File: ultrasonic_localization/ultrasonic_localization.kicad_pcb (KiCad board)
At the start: 2 copper layers, 69.6 x 80.4 mm, 212 parts, among them J101 USB_OTG_fix, J102 Conn_02x03_Odd_Even, J401 Screw_Terminal_1x02_Bat, Q101 BUK9Y29-40E, Q301 BC847, Q501 BC847, Q601 BC847, Q701 BC847, SW101 SW_Push, SW102 SW_DPDT, SW103 SW_DPDT, U101 ATMEGA32U4RC-AU, U102 MD0105, U103 4047, U201 nRF24L01+, U202 ANT016008LCS2442MA2, U301 LM324, U302 TCT40-16R/T, U401 AP3012, U402 AP3012, U403 TPS6223x, U404 LP5907SNX-3.3/NOPB, U405 BQ2423, U501 LM324, U502 TCT40-16R/T, U601 LM324, U602 TCT40-16R/T, U701 LM324, U702 TCT40-16R/T, U801 IMU, U802 Level_Shifter_4Channel, Y101 Crystal_GND24, Y201 16MHz

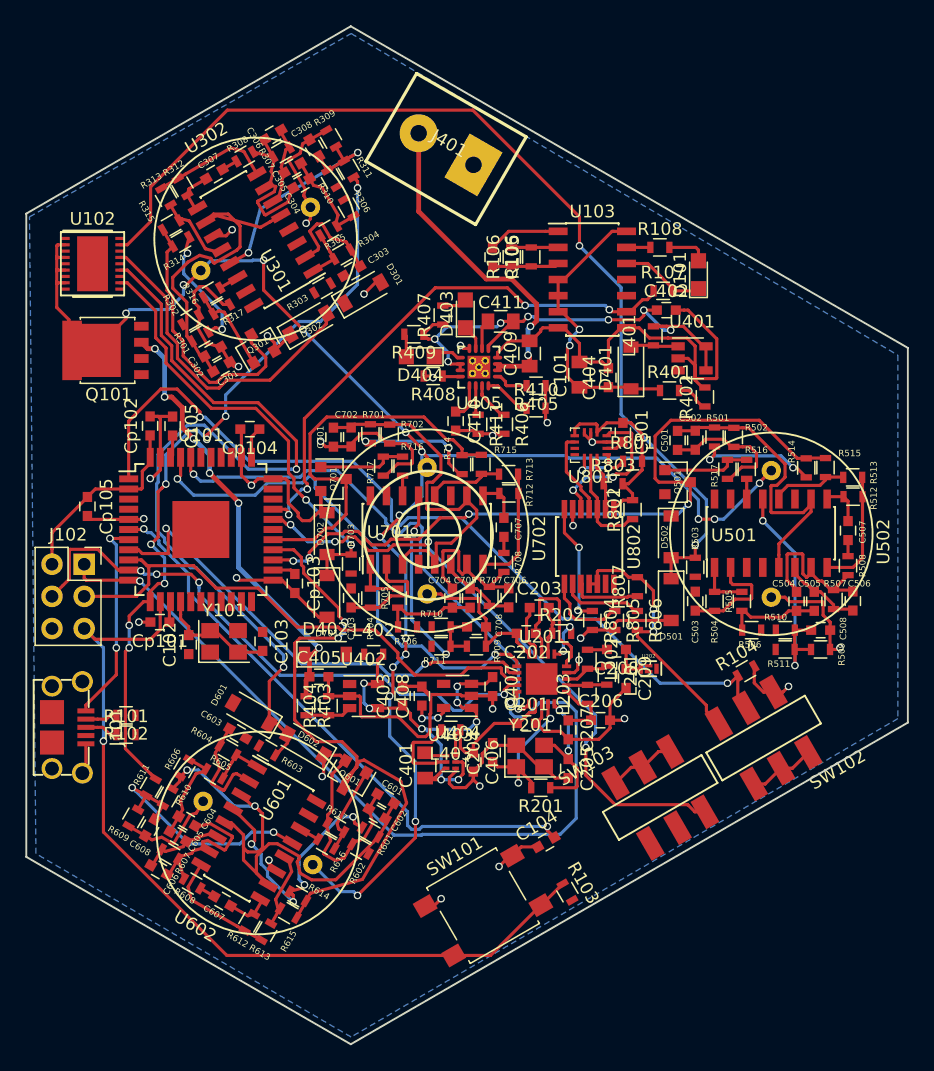
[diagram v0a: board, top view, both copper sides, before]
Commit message: Finished routing
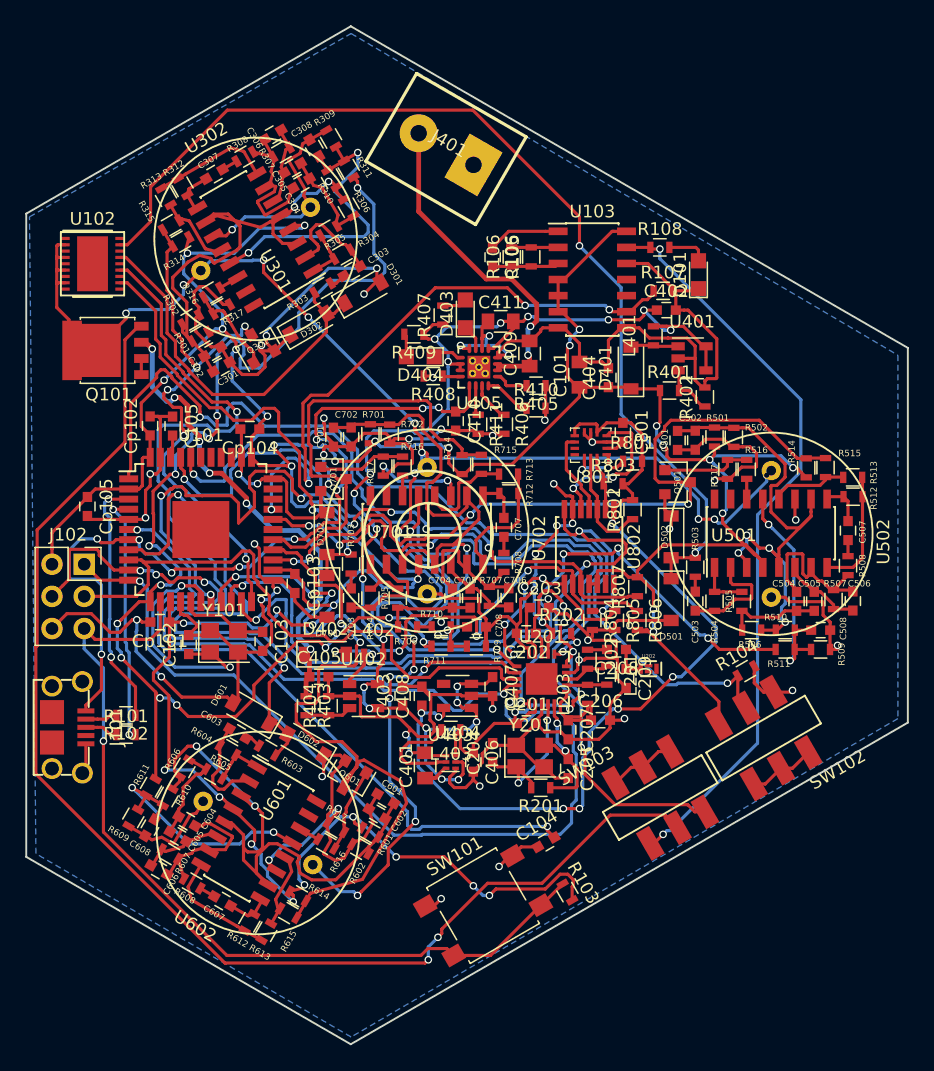
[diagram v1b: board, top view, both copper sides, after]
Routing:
- net +5V: track 117.0 -> 297.4 mm, vias 14 -> 34
- net GND: track 295.5 -> 438.4 mm, vias 28 -> 52
- net Net-(Q101-Pad4): track 0.00 -> 101.9 mm, vias 0 -> 2
- net /THRESH: track 60.5 -> 138.0 mm, vias 8 -> 17
- net /OSC_IC: track 1.88 -> 59.5 mm, vias 0 -> 2
- net /SCL: track 5.50 -> 62.1 mm, vias 0 -> 7
- net +1V8: track 18.8 -> 70.4 mm, vias 2 -> 7
- net /D2: track 9.67 -> 59.8 mm, vias 2 -> 4
- net /USB5V: track 19.2 -> 65.1 mm, vias 2 -> 10
- net /SDA: track 6.51 -> 52.3 mm, vias 0 -> 7
- net /D3: track 6.56 -> 44.2 mm, vias 0 -> 5
- net /Power/3V7: track 73.4 -> 104.3 mm, vias 15 -> 20
- net /SIG2: track 21.8 -> 43.2 mm, vias 0 -> 5
- net Net-(R101-Pad2): track 0.00 -> 20.0 mm, vias 0 -> 2
- net Net-(R102-Pad1): track 0.00 -> 19.9 mm, vias 0 -> 2
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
